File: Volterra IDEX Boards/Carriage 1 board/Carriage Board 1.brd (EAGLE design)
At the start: 84.5 x 61.3 mm, 20 parts, among them K1 FFC/FPC/34PIN/1MMPITCH/TOPLOCK, K2 Tool 0, X1 EXTDR-0, X4 24V, X5 X_LMT

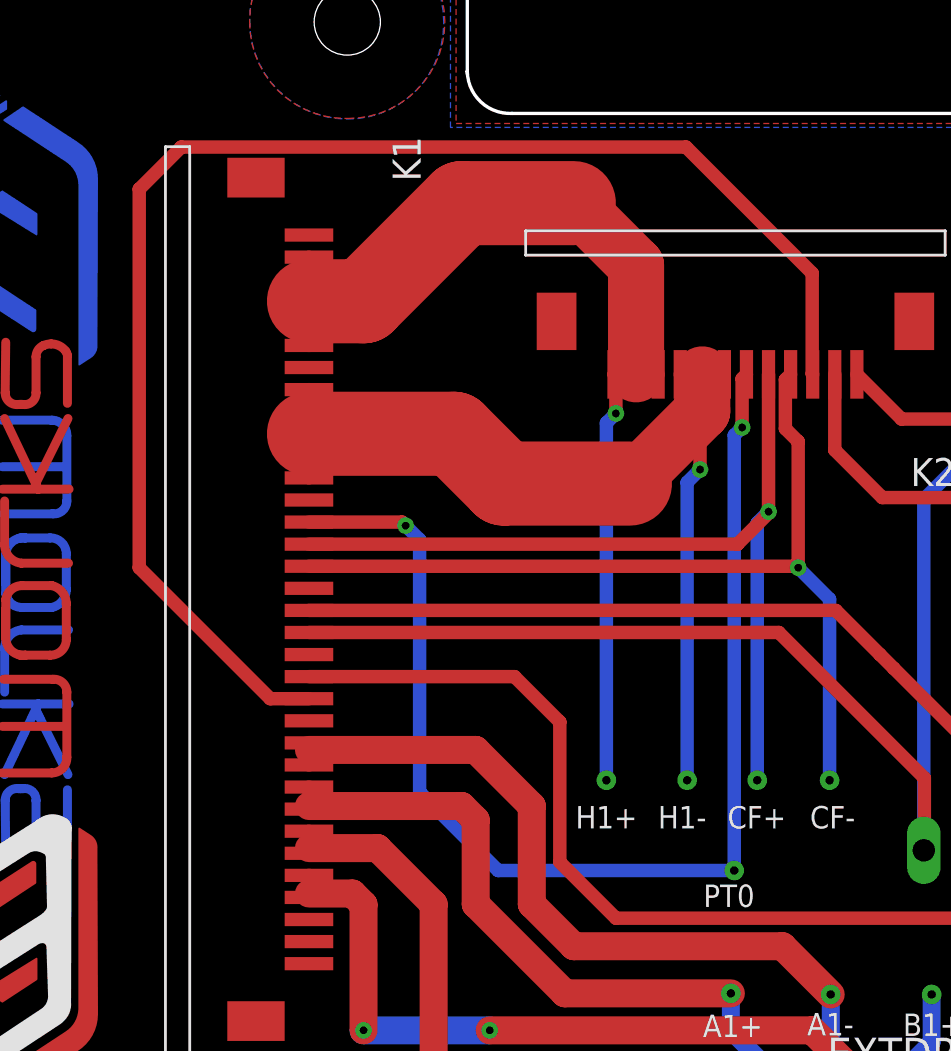
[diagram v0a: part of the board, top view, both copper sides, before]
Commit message: DRC checked of Chassis, Carriage 1 & 2, and created CAM files
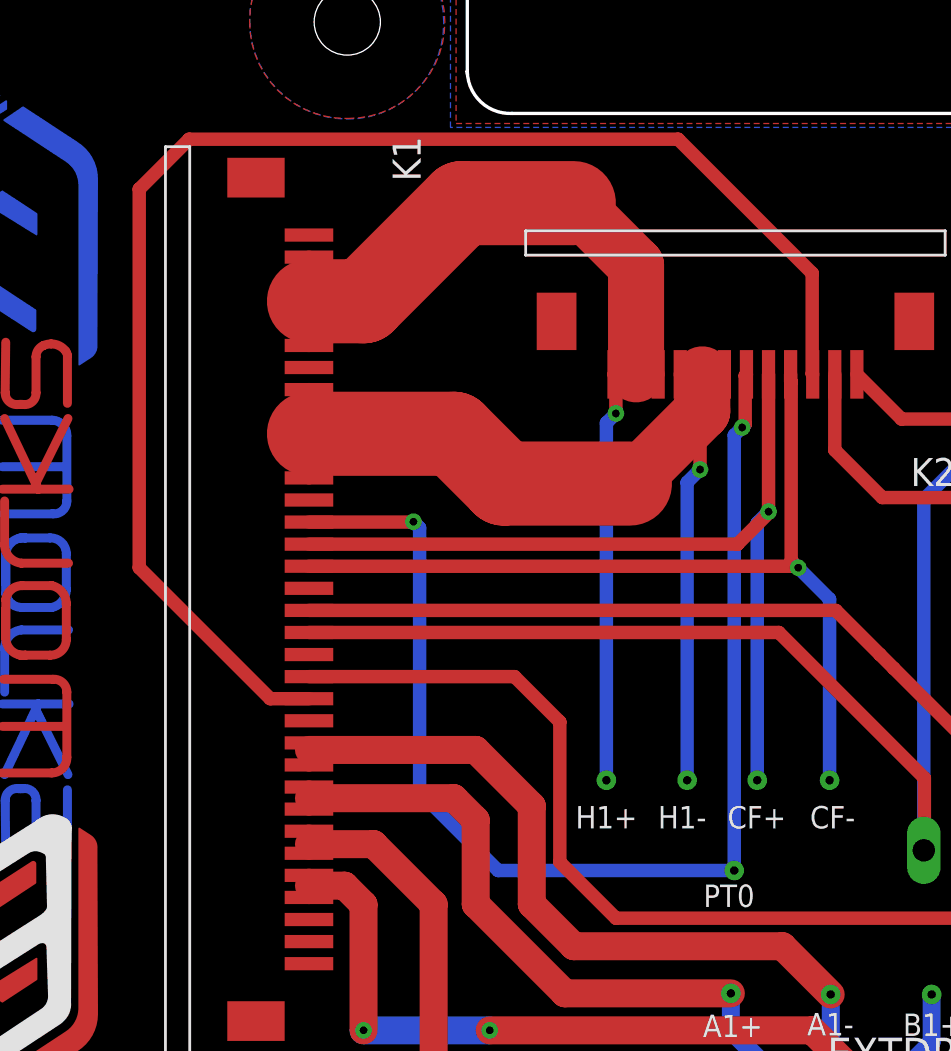
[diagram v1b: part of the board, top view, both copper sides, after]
